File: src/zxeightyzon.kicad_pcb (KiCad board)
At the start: 2 copper layers, 82.2 x 62 mm, 26 parts, among them J1 01x10, J2 01x10, J3 01x10, J4 Conn_02x02_Top_Bottom, U1 YM2149, U2 GAL22V10

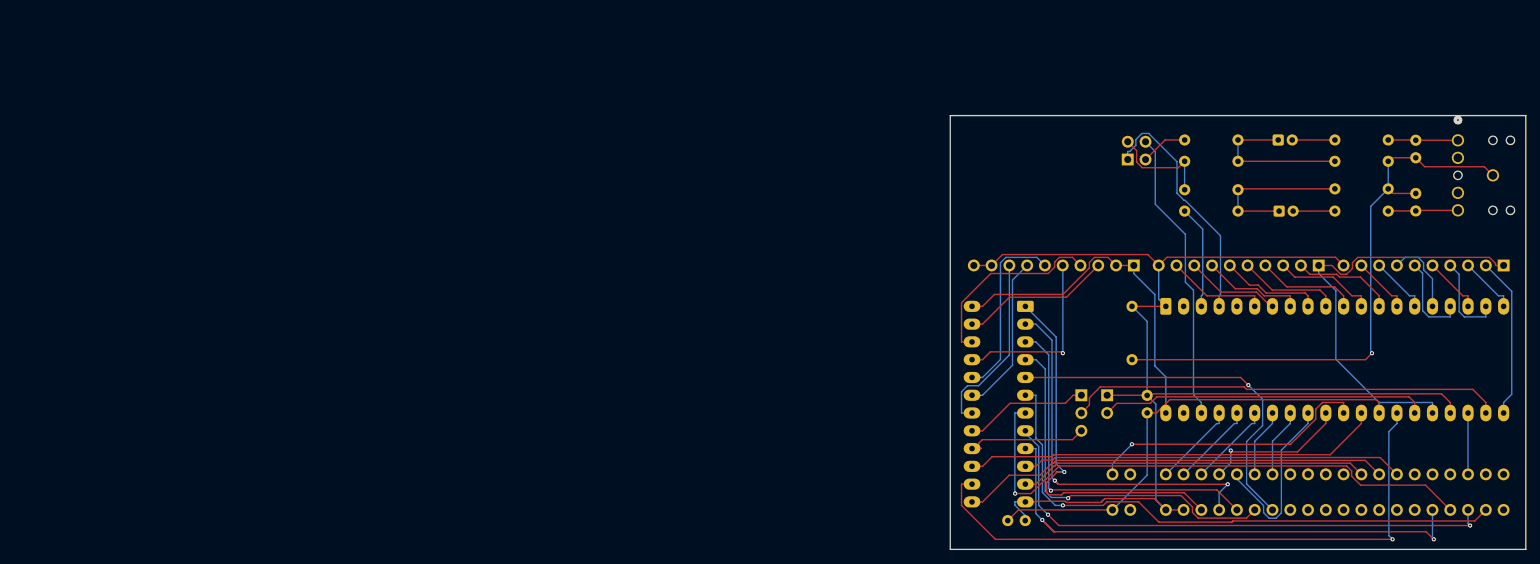
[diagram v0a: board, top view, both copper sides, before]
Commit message: fab files
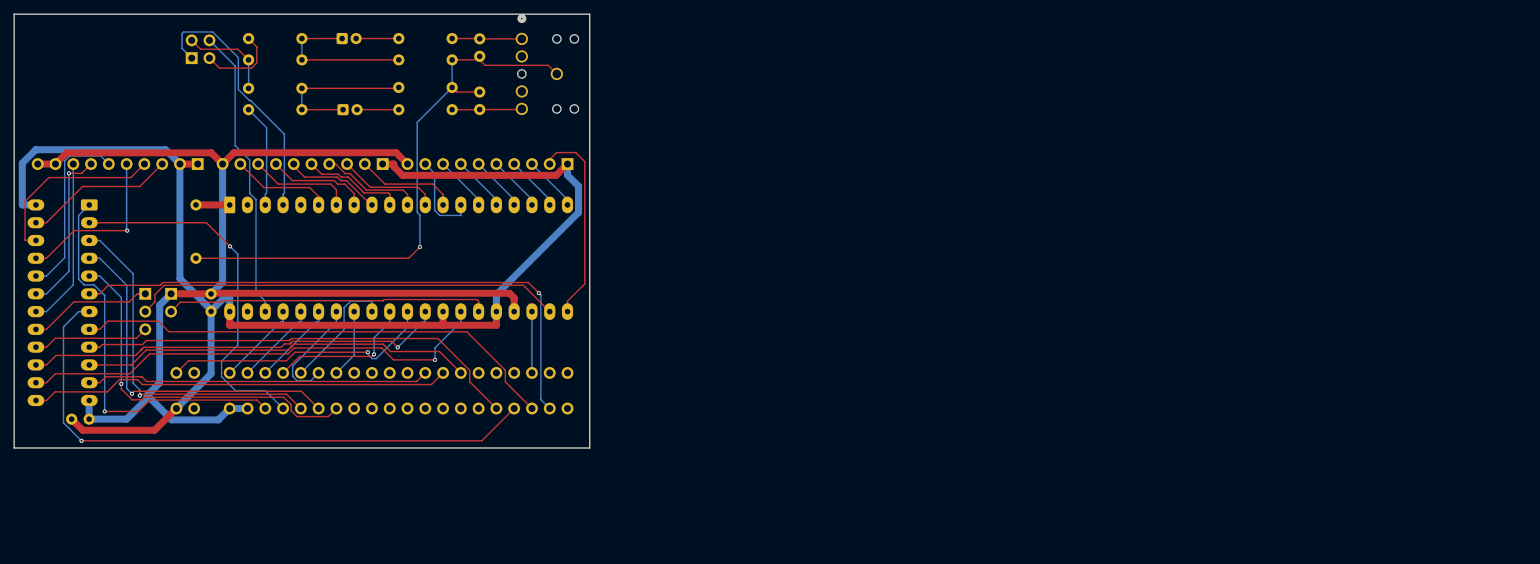
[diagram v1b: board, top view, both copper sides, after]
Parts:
- moved C2 134.5 mm to (84.9, 39.5)
- moved C6 134.5 mm to (46.2, 93.8)
- moved R6 134.5 mm to (93.0, 46.4)
- moved R7 134.5 mm to (93.0, 42.5)
- moved R8 134.5 mm to (93.0, 49.6)
- moved R9 134.5 mm to (93.0, 39.5)
- moved C3 134.5 mm to (104.5, 49.6)
- moved C4 134.5 mm to (104.5, 39.5)
- moved C5 134.5 mm to (66.2, 78.5)
- moved CO1 134.5 mm to (89.1, 89.8)
- moved FB1 134.5 mm to (64.0, 63.2)
- moved J2 134.5 mm to (90.7, 57.4)
- moved J3 134.5 mm to (64.3, 57.4)
- moved J4 134.5 mm to (63.4, 42.3)
- moved JP1 134.5 mm to (60.4, 75.9)
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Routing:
- net /A7: track 84.0 -> 63.9 mm, vias 2 -> 0
- net /BDIR: track 86.9 -> 68.2 mm
- net VCC: track 181.2 -> 194.2 mm
- net /D5: track 26.1 -> 17.8 mm
- net /A5: track 76.6 -> 69.9 mm, vias 2 -> 0
- net /D3: track 9.82 -> 16.3 mm
- net /IOA0: track 23.1 -> 29.0 mm
- net /A6: track 79.9 -> 85.7 mm
- net Net-(J4-Pin_2): track 6.75 -> 11.6 mm
- net /A0: track 57.0 -> 52.2 mm, vias 2 -> 1
- net /IOA4: track 12.7 -> 7.95 mm
- net /IOA2: track 12.7 -> 7.95 mm
- net /IOA7: track 8.38 -> 12.7 mm
- net /A2: track 54.6 -> 50.6 mm
- net /IOA5: track 11.4 -> 7.95 mm
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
